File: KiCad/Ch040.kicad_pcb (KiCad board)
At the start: 2 copper layers, 41.2 x 40 mm, 17 parts, among them J1 Conn_01x09, J2 Conn_01x09, J3 Conn_01x10, J4 Conn_01x02

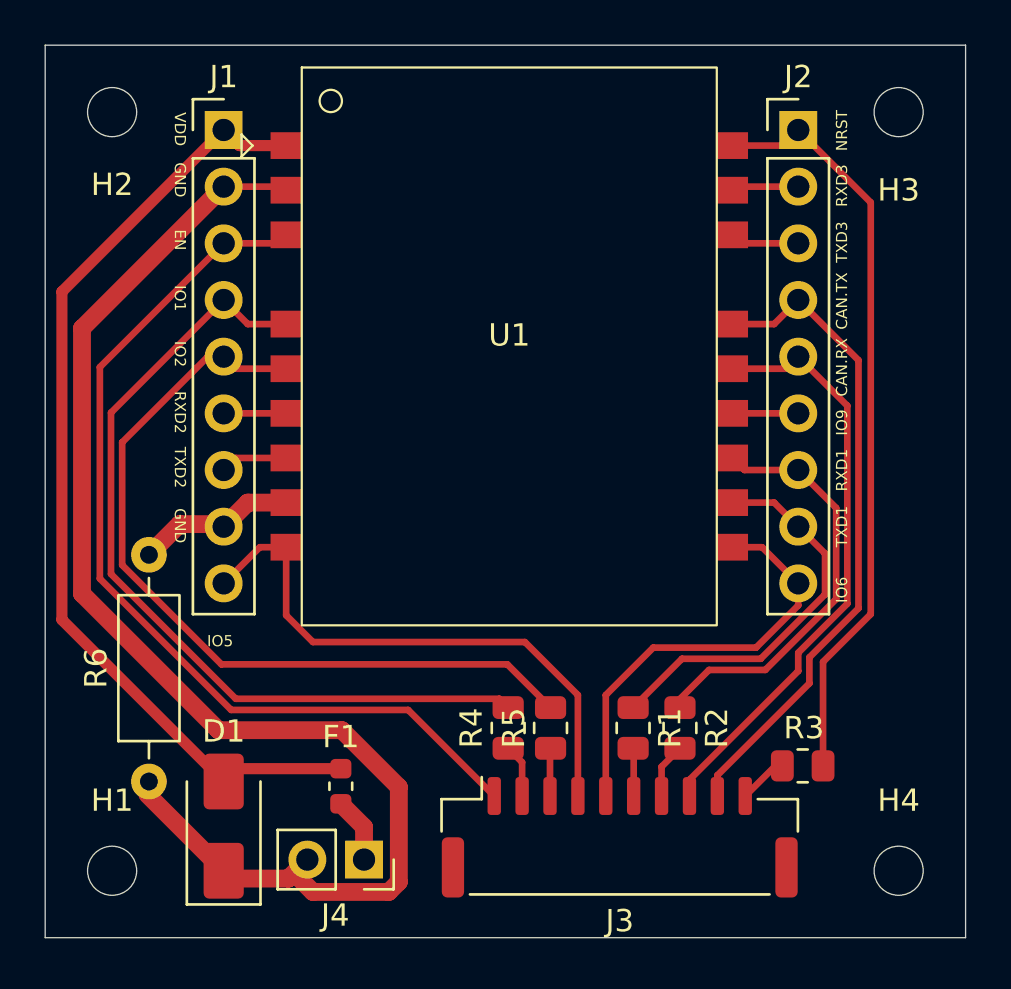
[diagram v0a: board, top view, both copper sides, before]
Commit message: Add files via upload
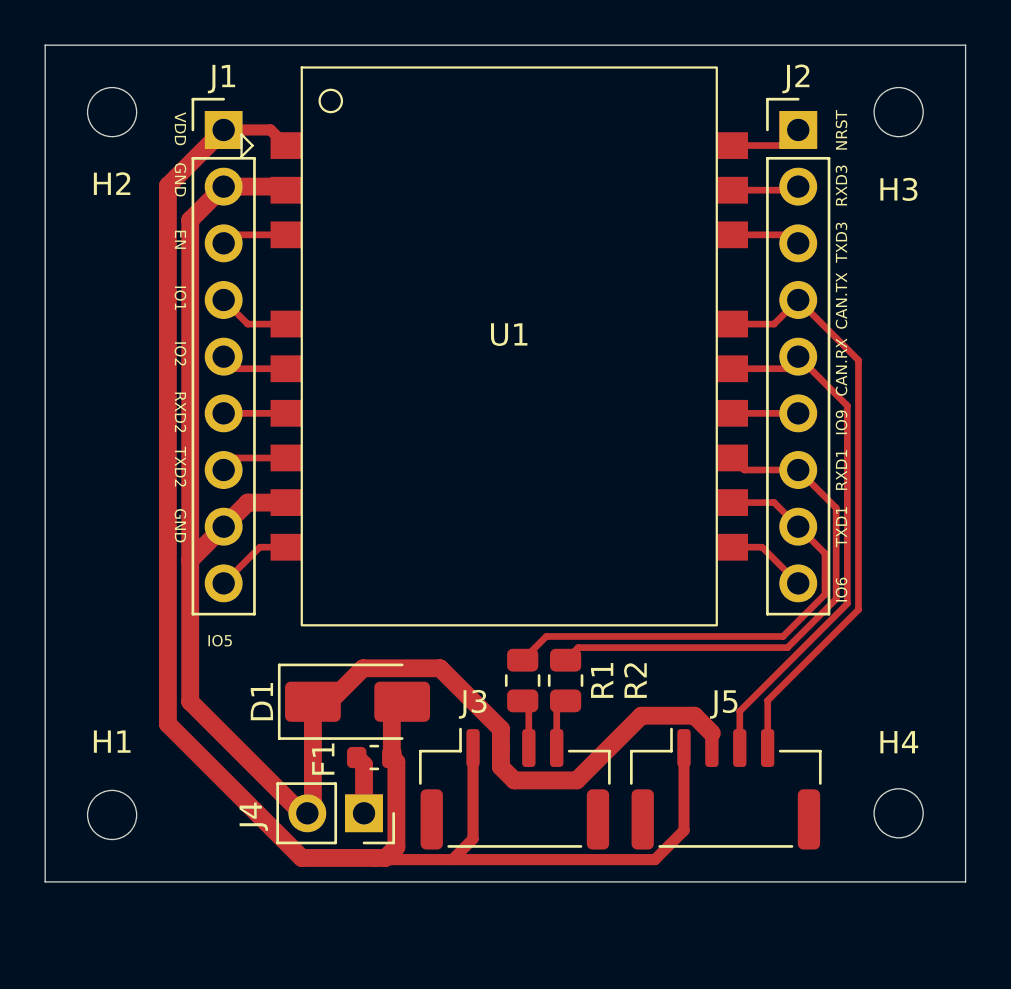
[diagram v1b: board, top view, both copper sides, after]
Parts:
- removed R3, R4, R5: 1k, Resistor_SMD:R_0805_2012Metric
- removed R6: R0, Resistor_THT:R_Axial_DIN0207_L6.3mm_D2.5mm_P10.16mm_Horizontal
- added J5: Conn_01x04, Connector_JST:JST_GH_SM04B-GHS-TB_1x04-1MP_P1.25mm_Horizontal, F.Cu at (142.8, 111.3)
- J3: value Conn_01x10 -> Conn_01x04; footprint Connector_JST:JST_GH_SM10B-GHS-TB_1x10-1MP_P1.25mm_Horizontal -> Connector_JST:JST_GH_SM04B-GHS-TB_1x04-1MP_P1.25mm_Horizontal
- moved D1 8.19 mm to (126.2, 107.4), turned to 0 degrees
- moved R2 5.55 mm to (135.6, 106.5)
- moved R1 5.39 mm to (133.7, 106.5)
- moved J3 5.17 mm to (133.3, 111.3)
- moved H4 2.58 mm to (150.5, 112.4)
- moved H1 2.50 mm to (115.2, 112.5)
- moved J4 2.08 mm to (126.5, 112.4)
- moved F1 1.98 mm to (127.0, 109.9), turned to 0 degrees
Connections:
- J1 pad 8: GND_LOCAL -> GND
- J3 pad 1: EN -> VDD
- J3 pad 2: IO1_EXT -> GND
- J3 pad 3: IO2_EXT -> UART1_TX
- J3 pad 4: IO5 -> UART1_RX
- U1 pad 8: GND_LOCAL -> GND
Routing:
- net EN: track 42.0 -> 2.96 mm
- net IO1: track 37.9 -> 3.25 mm
- net IO2: track 36.5 -> 3.02 mm
- net NRST: track 34.0 -> 3.24 mm
- net VDD: track 43.8 -> 74.0 mm
- net IO5: track 25.6 -> 3.47 mm
- net IO6: track 19.4 -> 3.62 mm
- net GND_LOCAL: track 7.21 -> 0.00 mm
- net GND: track 60.9 -> 68.1 mm
- net TXD1: track 17.6 -> 21.7 mm
- net RXD1: track 18.9 -> 22.9 mm
- net CAN_RX: track 26.7 -> 23.6 mm
- net CAN_TX: track 29.4 -> 26.3 mm
- net IO1_EXT: track 2.40 -> 0.00 mm
- net NRST_EXT: track 2.26 -> 0.00 mm
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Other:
- board size 41.2 x 40 mm -> 41.2 x 37.5 mm
